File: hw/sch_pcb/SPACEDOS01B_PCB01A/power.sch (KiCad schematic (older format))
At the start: 31 parts, among them J1 HEADER_2x01_PARALLEL, J2 HEADER_2x01_PARALLEL, J3 HEADER_2x01_PARALLEL, U6 TPS613221ADBV, U8 TPS613222ADBV

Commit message: edit
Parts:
- C22, C25, C32, C36, C38, C42, C48, C49, C50, C53, C54, C55: symbol SPACEDOS01A_PCB01A-rescue:C-device-DATALOGGER01A-rescue-CCP2019V01A-rescue -> SPACEDOS01B_PCB01A-rescue:C-device-DATALOGGER01A-rescue-CCP2019V01A-rescue-SPACEDOS01A_PCB01A-rescue
- C29, C45, C51, C52: symbol SPACEDOS01A_PCB01A-rescue:EMI_Filter_C-device-DATALOGGER01A-rescue-CCP2019V01A-rescue -> SPACEDOS01B_PCB01A-rescue:EMI_Filter_C-device-DATALOGGER01A-rescue-CCP2019V01A-rescue-SPACEDOS01A_PCB01A-rescue
- D1, D3: symbol SPACEDOS01A_PCB01A-rescue:D-device-DATALOGGER01A-rescue-CCP2019V01A-rescue -> SPACEDOS01B_PCB01A-rescue:D-device-DATALOGGER01A-rescue-CCP2019V01A-rescue-SPACEDOS01A_PCB01A-rescue
- F1, F2: symbol SPACEDOS01A_PCB01A-rescue:Polyfuse-device-DATALOGGER01A-rescue-CCP2019V01A-rescue -> SPACEDOS01B_PCB01A-rescue:Polyfuse-device-DATALOGGER01A-rescue-CCP2019V01A-rescue-SPACEDOS01A_PCB01A-rescue
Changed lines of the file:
@@
 EESchema Schematic File Version 4
-LIBS:SPACEDOS01A_PCB01A-cache
+LIBS:SPACEDOS01B_PCB01A-cache
 EELAYER 26 0
 EELAYER END
@@
 $EndDescr
 $Comp
-L SPACEDOS01A_PCB01A-rescue:D-device-DATALOGGER01A-rescue-CCP2019V01A-rescue D?
+L SPACEDOS01B_PCB01A-rescue:D-device-DATALOGGER01A-rescue-CCP2019V01A-rescue-SPACEDOS01A_PCB01A-rescue D?
 U 1 1 5C6BE250
 P 2800 1750
@@
 	2800 1950 2800 1900
 $Comp
-L SPACEDOS01A_PCB01A-rescue:EMI_Filter_C-device-DATALOGGER01A-rescue-CCP2019V01A-rescue C?
+L SPACEDOS01B_PCB01A-rescue:EMI_Filter_C-device-DATALOGGER01A-rescue-CCP2019V01A-rescue-SPACEDOS01A_PCB01A-rescue C?
 U 1 1 5C6BE26E
 P 3450 1650
@@
 $EndComp
 $Comp
-L SPACEDOS01A_PCB01A-rescue:C-device-DATALOGGER01A-rescue-CCP2019V01A-rescue C?
+L SPACEDOS01B_PCB01A-rescue:C-device-DATALOGGER01A-rescue-CCP2019V01A-rescue-SPACEDOS01A_PCB01A-rescue C?
 U 1 1 5C6BE27C
 P 3850 1750
@@
 	3450 1750 3450 1950
 $Comp
-L SPACEDOS01A_PCB01A-rescue:Polyfuse-device-DATALOGGER01A-rescue-CCP2019V01A-rescue F?
+L SPACEDOS01B_PCB01A-rescue:Polyfuse-device-DATALOGGER01A-rescue-CCP2019V01A-rescue-SPACEDOS01A_PCB01A-rescue F?
 U 1 1 5C6BE2A0
 P 2450 1550
@@
 	6750 3800 7100 3800
 $Comp
-L SPACEDOS01A_PCB01A-rescue:C-device-DATALOGGER01A-rescue-CCP2019V01A-rescue C?
+L SPACEDOS01B_PCB01A-rescue:C-device-DATALOGGER01A-rescue-CCP2019V01A-rescue-SPACEDOS01A_PCB01A-rescue C?
 U 1 1 5C6C450E
 P 8050 4050
@@
 $EndComp
 $Comp
-L SPACEDOS01A_PCB01A-rescue:C-device-DATALOGGER01A-rescue-CCP2019V01A-rescue C?
+L SPACEDOS01B_PCB01A-rescue:C-device-DATALOGGER01A-rescue-CCP2019V01A-rescue-SPACEDOS01A_PCB01A-rescue C?
 U 1 1 5C6C45C5
 P 8500 4050
@@
 Connection ~ 8500 3800
 $Comp
-L SPACEDOS01A_PCB01A-rescue:EMI_Filter_C-device-DATALOGGER01A-rescue-CCP2019V01A-rescue C?
+L SPACEDOS01B_PCB01A-rescue:EMI_Filter_C-device-DATALOGGER01A-rescue-CCP2019V01A-rescue-SPACEDOS01A_PCB01A-rescue C?
 U 1 1 5C6CDA68
 P 9050 3900
@@
 $EndComp
 $Comp
-L SPACEDOS01A_PCB01A-rescue:C-device-DATALOGGER01A-rescue-CCP2019V01A-rescue C?
+L SPACEDOS01B_PCB01A-rescue:C-device-DATALOGGER01A-rescue-CCP2019V01A-rescue-SPACEDOS01A_PCB01A-rescue C?
 U 1 1 5C6CDA6E
 P 9450 4000
@@
 	6750 5100 7100 5100
 $Comp
-L SPACEDOS01A_PCB01A-rescue:C-device-DATALOGGER01A-rescue-CCP2019V01A-rescue C?
+L SPACEDOS01B_PCB01A-rescue:C-device-DATALOGGER01A-rescue-CCP2019V01A-rescue-SPACEDOS01A_PCB01A-rescue C?
 U 1 1 5C6D0EB3
 P 8050 5350
@@
 $EndComp
 $Comp
-L SPACEDOS01A_PCB01A-rescue:C-device-DATALOGGER01A-rescue-CCP2019V01A-rescue C?
+L SPACEDOS01B_PCB01A-rescue:C-device-DATALOGGER01A-rescue-CCP2019V01A-rescue-SPACEDOS01A_PCB01A-rescue C?
 U 1 1 5C6D0EB9
 P 8500 5350
@@
 	8500 5200 8500 5100
 $Comp
-L SPACEDOS01A_PCB01A-rescue:C-device-DATALOGGER01A-rescue-CCP2019V01A-rescue C?
+L SPACEDOS01B_PCB01A-rescue:C-device-DATALOGGER01A-rescue-CCP2019V01A-rescue-SPACEDOS01A_PCB01A-rescue C?
 U 1 1 5C6D0EE7
 P 6300 5350
@@
 Connection ~ 8500 5100
 $Comp
-L SPACEDOS01A_PCB01A-rescue:EMI_Filter_C-device-DATALOGGER01A-rescue-CCP2019V01A-rescue C?
+L SPACEDOS01B_PCB01A-rescue:EMI_Filter_C-device-DATALOGGER01A-rescue-CCP2019V01A-rescue-SPACEDOS01A_PCB01A-rescue C?
 U 1 1 5C6D0EF9
 P 9050 5200
@@
 $EndComp
 $Comp
-L SPACEDOS01A_PCB01A-rescue:C-device-DATALOGGER01A-rescue-CCP2019V01A-rescue C?
+L SPACEDOS01B_PCB01A-rescue:C-device-DATALOGGER01A-rescue-CCP2019V01A-rescue-SPACEDOS01A_PCB01A-rescue C?
 U 1 1 5C6D0EFF
 P 9450 5300
@@
 	2000 1550 2150 1550
 $Comp
-L SPACEDOS01A_PCB01A-rescue:D-device-DATALOGGER01A-rescue-CCP2019V01A-rescue D?
+L SPACEDOS01B_PCB01A-rescue:D-device-DATALOGGER01A-rescue-CCP2019V01A-rescue-SPACEDOS01A_PCB01A-rescue D?
 U 1 1 5C589333
 P 2800 3550
@@
 	2800 3750 2800 3700
 $Comp
-L SPACEDOS01A_PCB01A-rescue:EMI_Filter_C-device-DATALOGGER01A-rescue-CCP2019V01A-rescue C?
+L SPACEDOS01B_PCB01A-rescue:EMI_Filter_C-device-DATALOGGER01A-rescue-CCP2019V01A-rescue-SPACEDOS01A_PCB01A-rescue C?
 U 1 1 5C589354
 P 3450 3450
@@
 $EndComp
 $Comp
-L SPACEDOS01A_PCB01A-rescue:C-device-DATALOGGER01A-rescue-CCP2019V01A-rescue C?
+L SPACEDOS01B_PCB01A-rescue:C-device-DATALOGGER01A-rescue-CCP2019V01A-rescue-SPACEDOS01A_PCB01A-rescue C?
 U 1 1 5C589368
 P 3850 3550
@@
 	3450 3550 3450 3750
 $Comp
-L SPACEDOS01A_PCB01A-rescue:Polyfuse-device-DATALOGGER01A-rescue-CCP2019V01A-rescue F?
+L SPACEDOS01B_PCB01A-rescue:Polyfuse-device-DATALOGGER01A-rescue-CCP2019V01A-rescue-SPACEDOS01A_PCB01A-rescue F?
 U 1 1 5C58939A
 P 2450 3350
@@
 	4200 1550 4200 1500
 $Comp
-L SPACEDOS01A_PCB01A-rescue:C-device-DATALOGGER01A-rescue-CCP2019V01A-rescue C?
+L SPACEDOS01B_PCB01A-rescue:C-device-DATALOGGER01A-rescue-CCP2019V01A-rescue-SPACEDOS01A_PCB01A-rescue C?
 U 1 1 5C5FA3D4
 P 3100 1750
@@
 $EndComp
 $Comp
-L SPACEDOS01A_PCB01A-rescue:C-device-DATALOGGER01A-rescue-CCP2019V01A-rescue C?
+L SPACEDOS01B_PCB01A-rescue:C-device-DATALOGGER01A-rescue-CCP2019V01A-rescue-SPACEDOS01A_PCB01A-rescue C?
 U 1 1 5C5FB0D4
 P 3100 3550
@@
 $EndComp
 $Comp
-L SPACEDOS01A_PCB01A-rescue:C-device-DATALOGGER01A-rescue-CCP2019V01A-rescue C?
+L SPACEDOS01B_PCB01A-rescue:C-device-DATALOGGER01A-rescue-CCP2019V01A-rescue-SPACEDOS01A_PCB01A-rescue C?
 U 1 1 5C6C894E
 P 6300 4050

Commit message: edit
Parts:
- removed C22, C38, C49: 10uF, Mlab_R:SMD-0805, symbol SPACEDOS01B_PCB01A-rescue:C-device-DATALOGGER01A-rescue-CCP2019V01A-rescue-SPAC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
- removed C25, C48, C53: 100nF, Mlab_R:SMD-0805, symbol SPACEDOS01B_PCB01A-rescue:C-device-DATALOGGER01A-rescue-CCP2019V01A-rescue-SPAC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
- removed C45, C51: NFM21PC105-1uF, Mlab_L:FIR1, symbol SPACEDOS01B_PCB01A-rescue:EMI_Filter_C-device-DATALOGGER01A-rescue-CCP2019V01A-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
- removed D1: BZV55C-5,6V, Diode_SMD:D_MiniMELF, symbol SPACEDOS01B_PCB01A-rescue:D-device-DATALOGGER01A-rescue-CCP2019V01A-rescue-SPAC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
- removed F1: SR010-15 100mA, Mlab_R:SMD-0805, symbol SPACEDOS01B_PCB01A-rescue:Polyfuse-device-DATALOGGER01A-rescue-CCP2019V01A-resc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
- removed L2: DFE252012P-4R7M, Resistor_SMD:R_0805_2012Metric_Pad1.15x1.40mm_HandSolder, symbol Device:L_Small
- removed R24, R25, R27: -, Mlab_R:SMD-0805, symbol Device:R
- removed R28: 0R, Mlab_R:SMD-0805, symbol Device:R
- removed U6: TPS613221ADBV, Package_TO_SOT_SMD:SOT-23-5, symbol MLAB_IO:TPS61322xA
- F2: symbol SPACEDOS01B_PCB01A-rescue:Polyfuse-device-DATALOGGER01A-rescue-CCP2019V01A-rescue-SPACEDOS01A_PCB01A-rescue -> SPACEDOS01B_PCB01A-rescue:Polyfuse-device-DATALOGGER01A-rescue-CCP2019V01A-rescue-SPACEDOS01A_PCB01A-rescue-SPACEDOS01B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
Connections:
- net labels removed: 5
- wire segments 74 -> 35
- no-connect marks 0 -> 1
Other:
- moved on the sheet: C32, C42, C50, C52, C54, J1, L3, U8

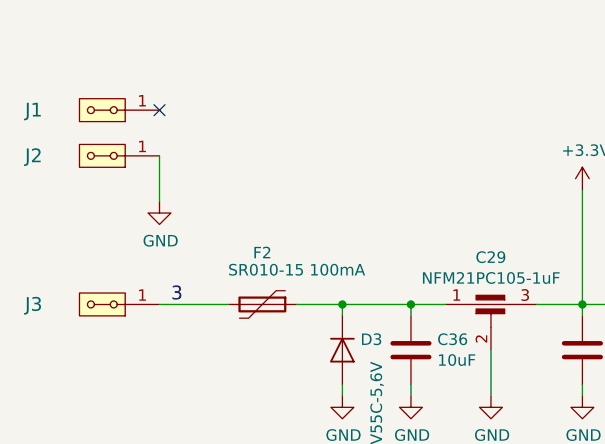
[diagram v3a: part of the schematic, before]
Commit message: edit
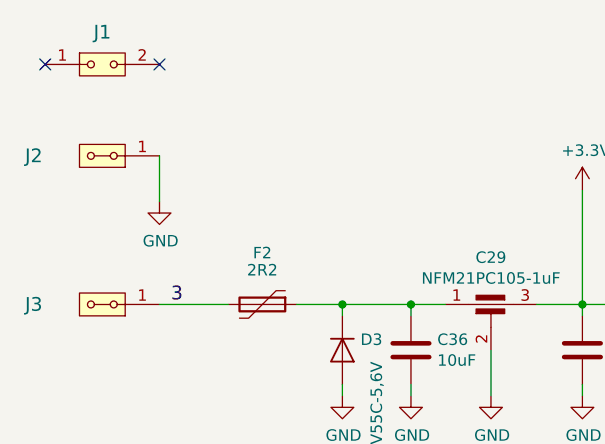
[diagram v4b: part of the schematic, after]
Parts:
- removed J1: HEADER_2x01_PARALLEL, Mlab_Pin_Headers:Straight_1x02, symbol MLAB_HEADER:HEADER_2x01_PARALLEL
- added J1: HEADER_2x01, Mlab_Pin_Headers:Straight_1x02, symbol MLAB_HEADER:HEADER_2x01
- C29, C52: footprint Mlab_L:FIR1 -> Mlab_L:FIR_0805
- F2: value SR010-15 100mA -> 2R2
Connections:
- no-connect marks 1 -> 2
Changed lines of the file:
@@
 EESchema Schematic File Version 4
 LIBS:SPACEDOS01B_PCB01A-cache
-EELAYER 29 0
+EELAYER 26 0
 EELAYER END
 $Descr A4 11693 8268
@@
 F 0 "C52" H 8950 3705 50  0000 C CNN
 F 1 "NFM21PC105-1uF" H 8950 3614 50  0000 C CNN
-F 2 "Mlab_L:FIR1" V 8950 3400 50  0001 C CNN
+F 2 "Mlab_L:FIR_0805" V 8950 3400 50  0001 C CNN
 F 3 "http://www.murata.com/~/media/webrenewal/support/library/catalog/products/emc/emifil/c31e.ashx?la=en-gb" V 8950 3400 50  0001 C CNN
 	1    8950 3400
@@
 Wire Wire Line
 	8950 3500 8950 3800
-$Comp
-L MLAB_HEADER:HEADER_2x01_PARALLEL J1
-U 1 1 5C5733E7
-P 1750 2500
-F 0 "J1" H 2050 2500 60  0000 C CNN
-F 1 "HEADER_2x01_PARALLEL" H 1667 2369 60  0001 C CNN
-F 2 "Mlab_Pin_Headers:Straight_1x02" H 1750 2500 60  0001 C CNN
-F 3 "" H 1750 2500 60  0000 C CNN
-	1    1750 2500
-	-1   0    0    1
-$EndComp
 $Comp
 L SPACEDOS01B_PCB01A-rescue:D-device-DATALOGGER01A-rescue-CCP2019V01A-rescue-SPACEDOS01A_PCB01A-rescue D?
@@
 F 0 "C29" H 3450 3755 50  0000 C CNN
 F 1 "NFM21PC105-1uF" H 3450 3664 50  0000 C CNN
-F 2 "Mlab_L:FIR1" V 3450 3450 50  0001 C CNN
+F 2 "Mlab_L:FIR_0805" V 3450 3450 50  0001 C CNN
 F 3 "http://www.murata.com/~/media/webrenewal/support/library/catalog/products/emc/emifil/c31e.ashx?la=en-gb" V 3450 3450 50  0001 C CNN
 	1    3450 3450
@@
 AR Path="/5C69BCB4/5C58939A" Ref="F2"  Part="1"
 F 0 "F2" V 2225 3350 50  0000 C CNN
-F 1 "SR010-15 100mA " V 2300 3500 50  0000 C CNN
+F 1 "2R2" V 2300 3350 50  0000 C CNN
 F 2 "Mlab_R:SMD-0805" H 2500 3150 50  0001 L CNN
 F 3 "" H 2450 3350 50  0001 C CNN
@@
 Wire Wire Line
 	2000 3350 2300 3350
-NoConn ~ 2000 2500
+$Comp
+L MLAB_HEADER:HEADER_2x01 J1
+U 1 1 5C82097F
+P 1750 2300
+F 0 "J1" H 1750 2441 60  0000 C CNN
+F 1 "HEADER_2x01" H 1750 2441 60  0001 C CNN
+F 2 "Mlab_Pin_Headers:Straight_1x02" H 1750 2300 60  0001 C CNN
+F 3 "" H 1750 2300 60  0000 C CNN
+	1    1750 2300
+	1    0    0    -1
+$EndComp
+NoConn ~ 1500 2300
+NoConn ~ 2000 2300
 $EndSCHEMATC
